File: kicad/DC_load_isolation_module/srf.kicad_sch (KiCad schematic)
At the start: 34 parts, among them Q1 MMBT5551L, Q26 MMBT5551L, Q27 MMBT5551L, Q28 MMBT5551L, Q29 MMBT5551L, T2 UMEC_UT20A13S

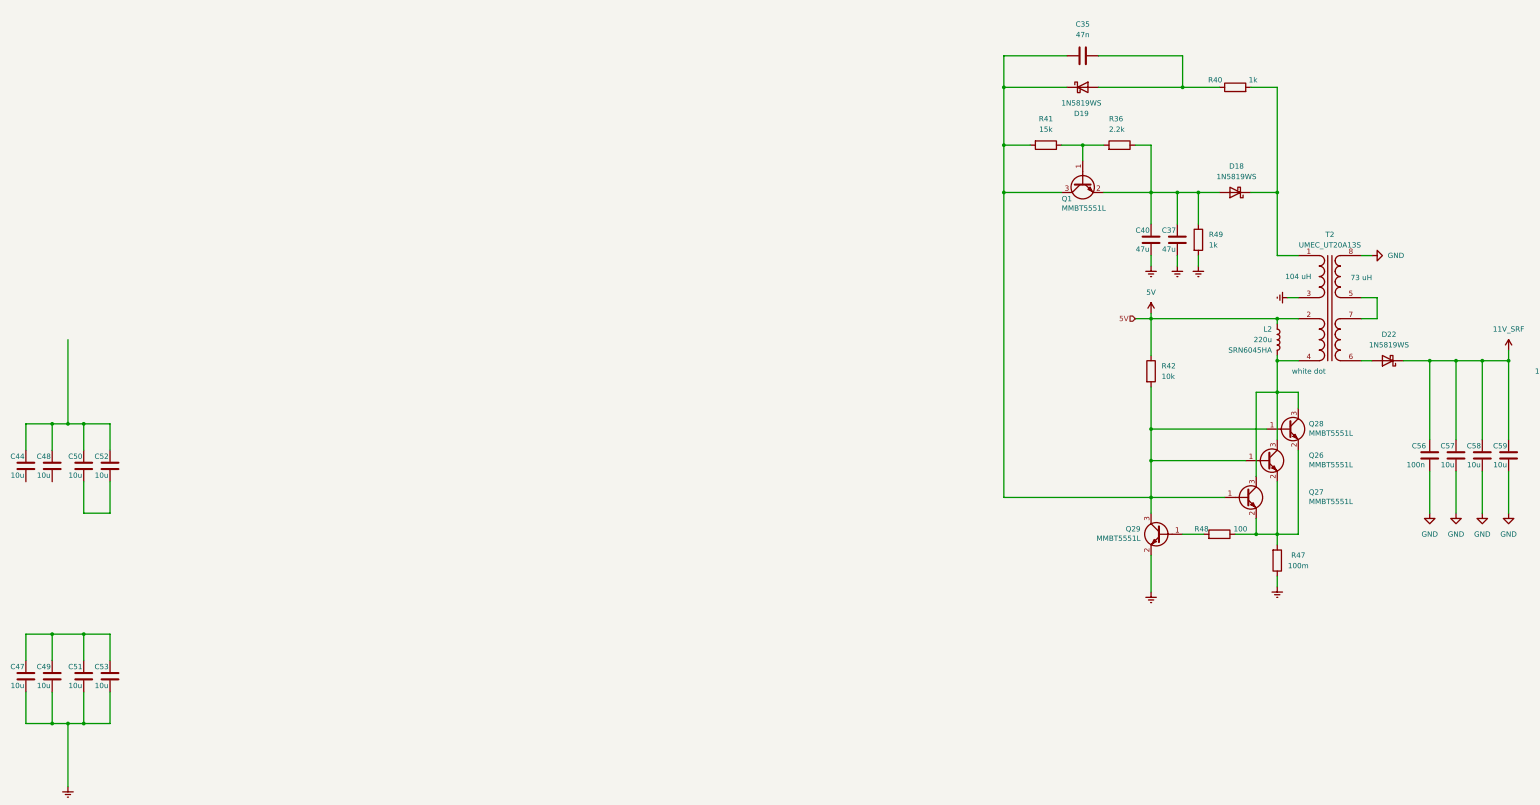
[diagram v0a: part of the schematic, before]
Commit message: Working on layout.
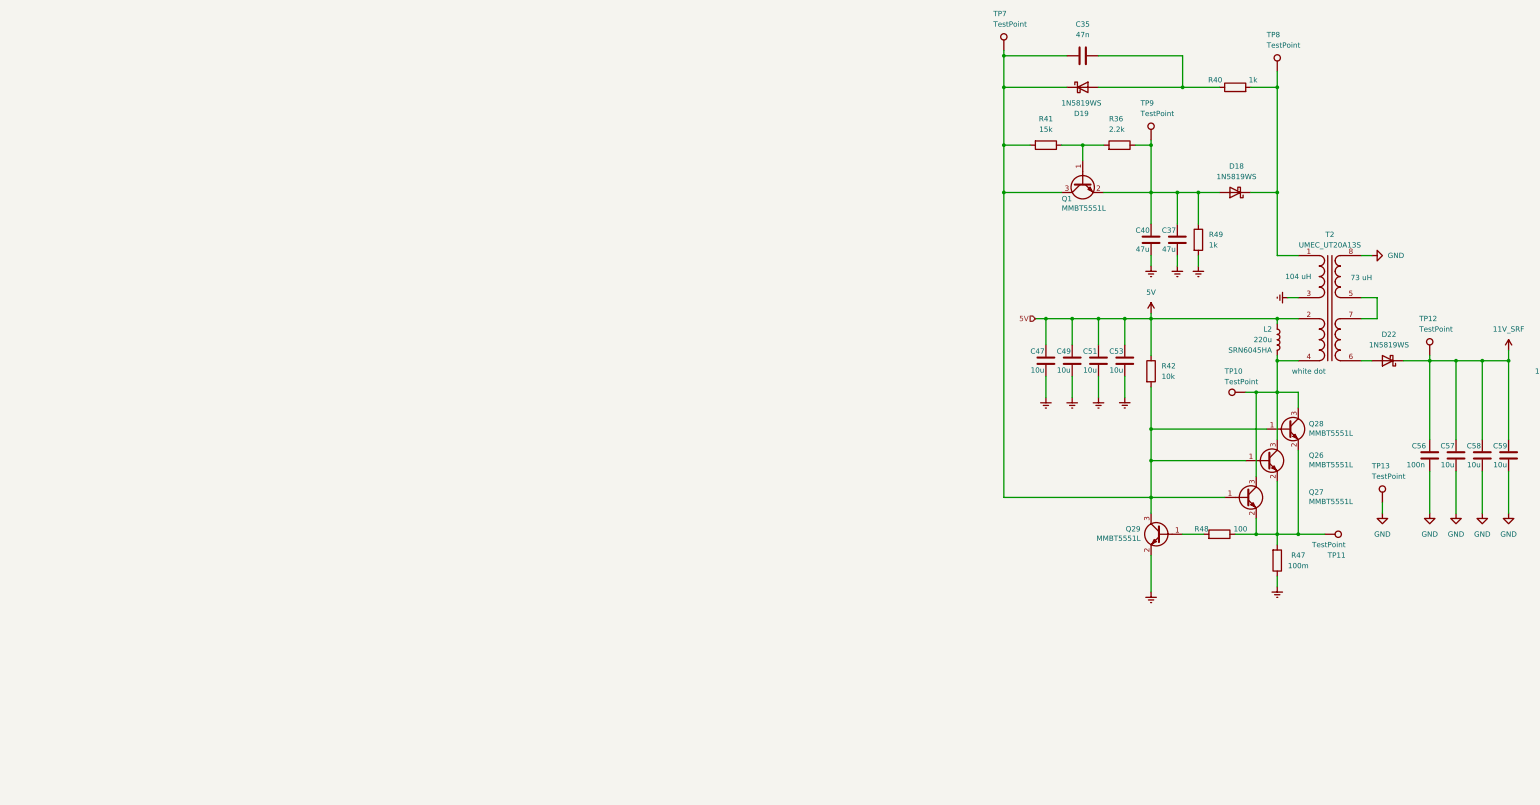
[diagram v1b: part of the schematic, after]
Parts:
- removed C44, C48, C50, C52: 10u, Capacitor_SMD:C_0603_1608Metric_Pad1.08x0.95mm_HandSolder, symbol Device:C
- added TP10, TP11, TP12, TP13, TP7, TP8, TP9: TestPoint, TestPoint:TestPoint_Pad_D2.0mm, symbol Connector:TestPoint
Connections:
- net 11V_SRF: now also TP12.1
- net 5V: now also C47.1, C49.1, C51.1, C53.1
- net GND: now also TP13.1
- net at D18.1 (K), R40.2, T2.1 (AA): now also TP8.1
- net at L2.1, Q26.3 (C), Q27.3 (C)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: now also TP10.1
- net at C35.1, D19.1 (K), Q1.3 (C)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: now also TP7.1
- net at Q26.2 (E), Q27.2 (E), Q28.2 (E)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: now also TP11.1
- net at C37.1, C40.1, D18.2 (A)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: now also TP9.1
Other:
- moved on the sheet: C47, C49, C51, C53
